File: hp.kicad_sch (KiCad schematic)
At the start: 3 parts, among them J9 Screw_Terminal_01x02

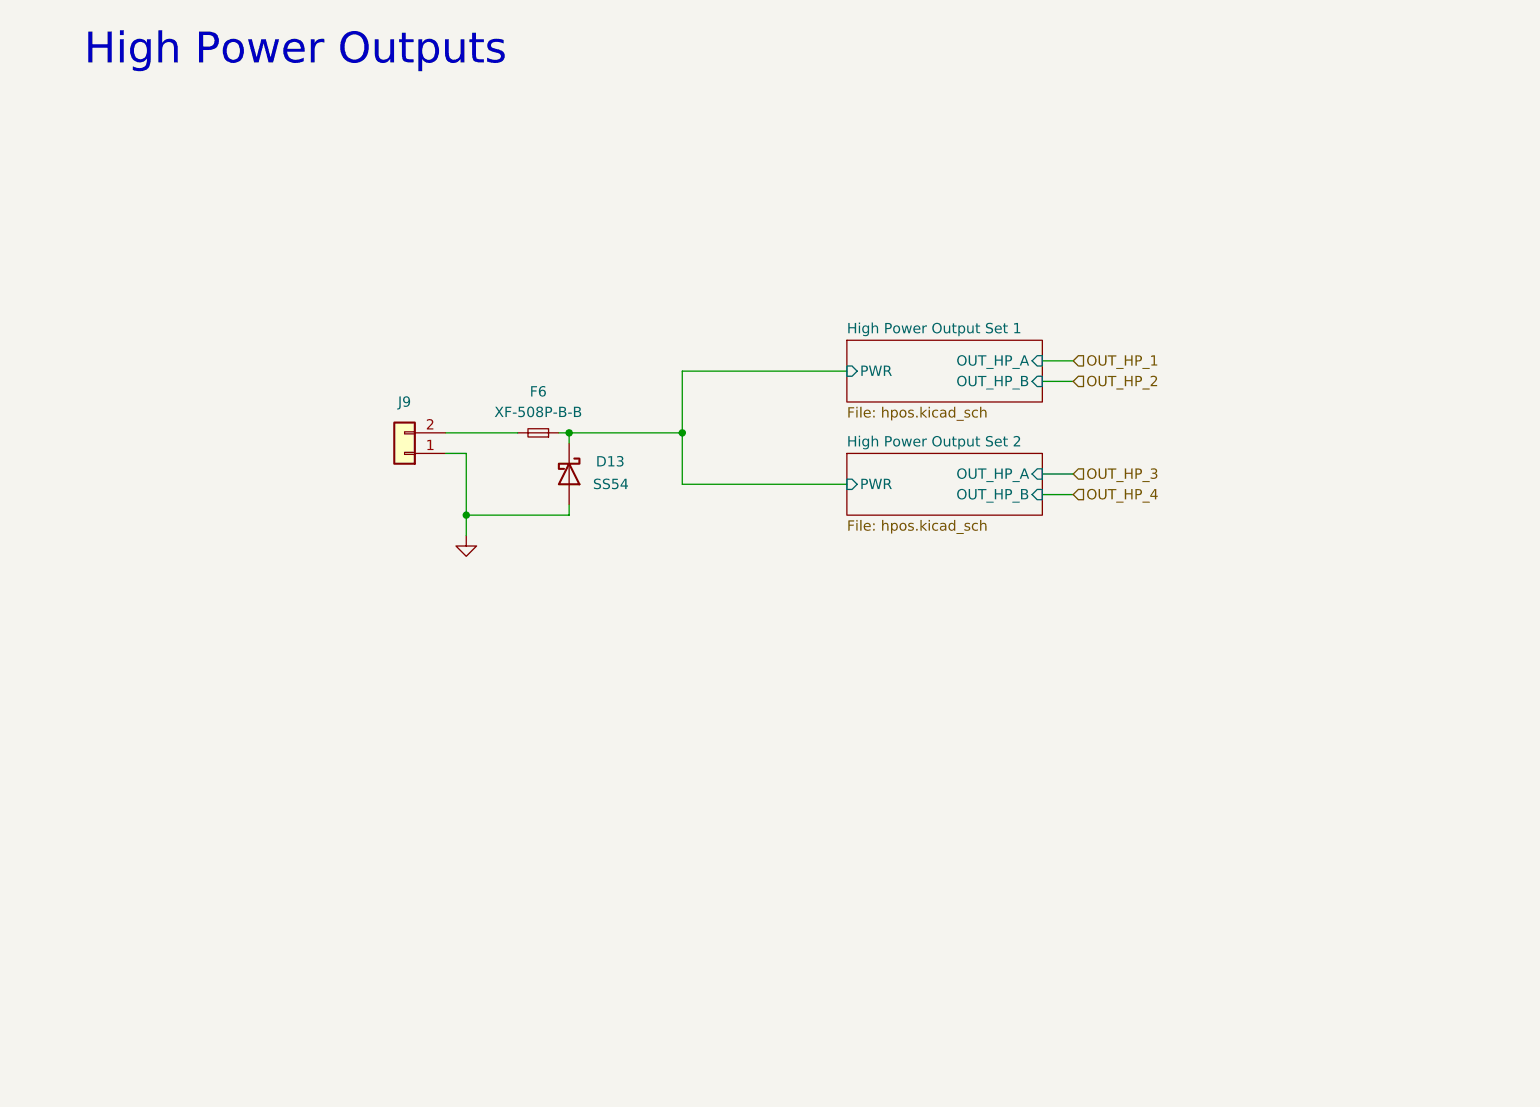
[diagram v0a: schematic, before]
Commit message: ???
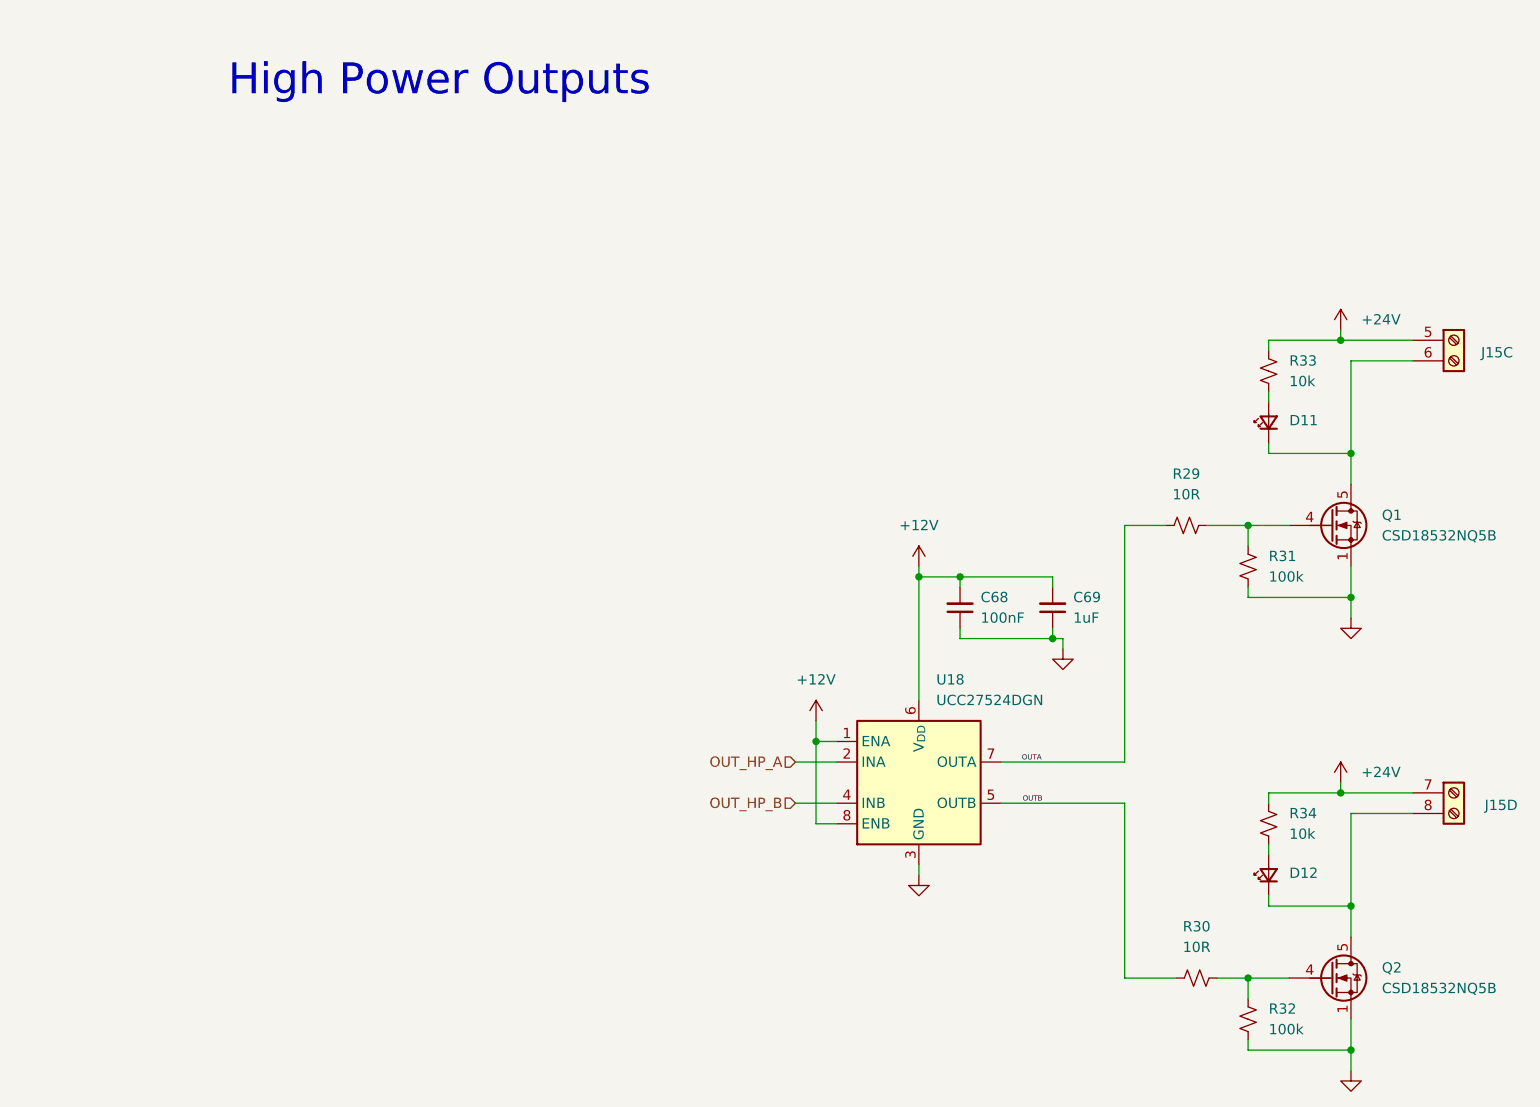
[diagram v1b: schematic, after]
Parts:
- removed D13: SS54, Diode_SMD:D_SMA, symbol Diode:SS38
- removed F6: XF-508P-B-B, Fuse:Fuseholder_Blade_Mini_Keystone_3568, symbol Device:Fuse_Small
- removed J9: Screw_Terminal_01x02, Connector_Phoenix_MSTB:PhoenixContact_MSTBA_2,5_2-G_1x02_P5.00mm_Horizontal, symbol Connector_Generic:Conn_01x02
- added C68: 100nF, APRLPrints:C_0603, symbol Device:C_Small
- added C69: 1uF, APRLPrints:C_0603, symbol Device:C_Small
- added D11, D12: LED_Small, APRLPrints:LED_0603, symbol Device:LED_Small
- added J15: Screw_Terminal_06x01x02, TerminalBlock_Ningbo-Kagnex:TerminalBlock_Ningbo-Kagnex_HB9500M_1x12_P9.5mm, symbol libserie:Screw_Terminal_06x01x02
- added Q1, Q2: CSD18532NQ5B, Package_TO_SOT_SMD:TDSON-8-1, symbol Transistor_FET:CSD18532NQ5B
- added R29, R30: 10R, APRLPrints:R_0603, symbol Device:R_Small_US
- added R31, R32: 100k, APRLPrints:R_0603, symbol Device:R_Small_US
- added R33, R34: 10k, APRLPrints:R_0603, symbol Device:R_Small_US
- added U18: UCC27524DGN, Package_SO:Texas_DGN0008G_VSSOP-8-1EP_3x3mm_P0.65mm_EP2x2.94mm_Mask1.846x2.15mm_ThermalVias, symbol Driver_FET:UCC27524DGN
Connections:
- net GND: now also C68.1, C69.1, Q1.1 (S), Q1.2 (S), Q1.3 (S), Q2.1 (S), Q2.2 (S), Q2.3 (S), R31.1, R32.1, U18.3 (GND), U18.9 (GND)
- new net: Q2.4 (G), R30.2, R32.2
- new net: D12.1 (K), J15.8 (Pin_2), Q2.5 (D)
- new net: D11.1 (K), J15.6 (Pin_2), Q1.5 (D)
- new net: D11.2 (A), R33.2
- new net: D12.2 (A), R34.2
- new net: Q1.4 (G), R29.2, R31.2
- new net +12V: C68.2, C69.2, U18.1 (ENA), U18.6 (V_{DD}), U18.8 (ENB)
- new net +24V: J15.5 (Pin_1), J15.7 (Pin_1), R33.1, R34.1
- new net OUTA: R29.1, U18.7 (OUTA)
- new net OUTB: R30.1, U18.5 (OUTB)
- new net OUT_HP_A: U18.2 (INA)
- new net OUT_HP_B: U18.4 (INB)
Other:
- removed sheet High Power Output Set 1
- removed sheet High Power Output Set 2
